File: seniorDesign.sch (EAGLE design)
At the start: 23 parts, among them Q1 mmbt2222, Q2 mmbt2222, Q3 BSS138, U1 TCS34725, X2 ESP-12

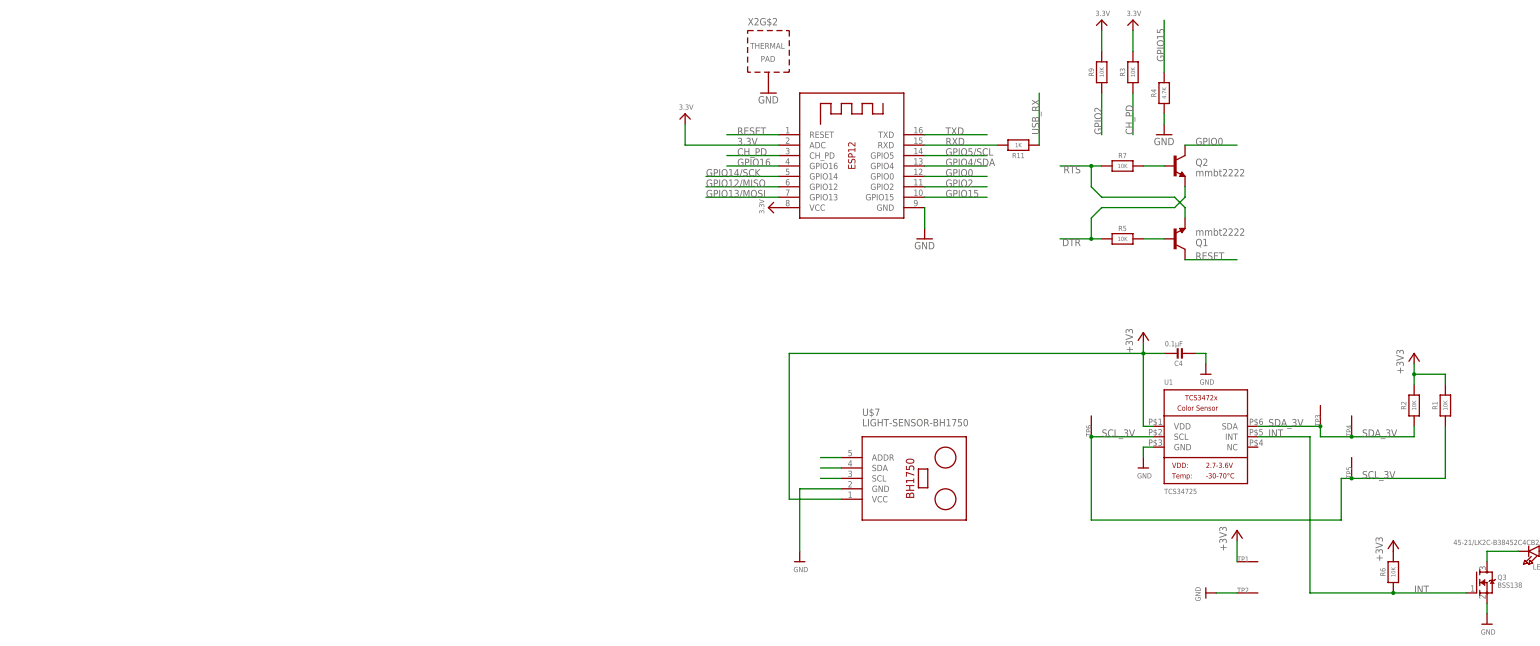
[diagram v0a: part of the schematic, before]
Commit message: Add files via upload
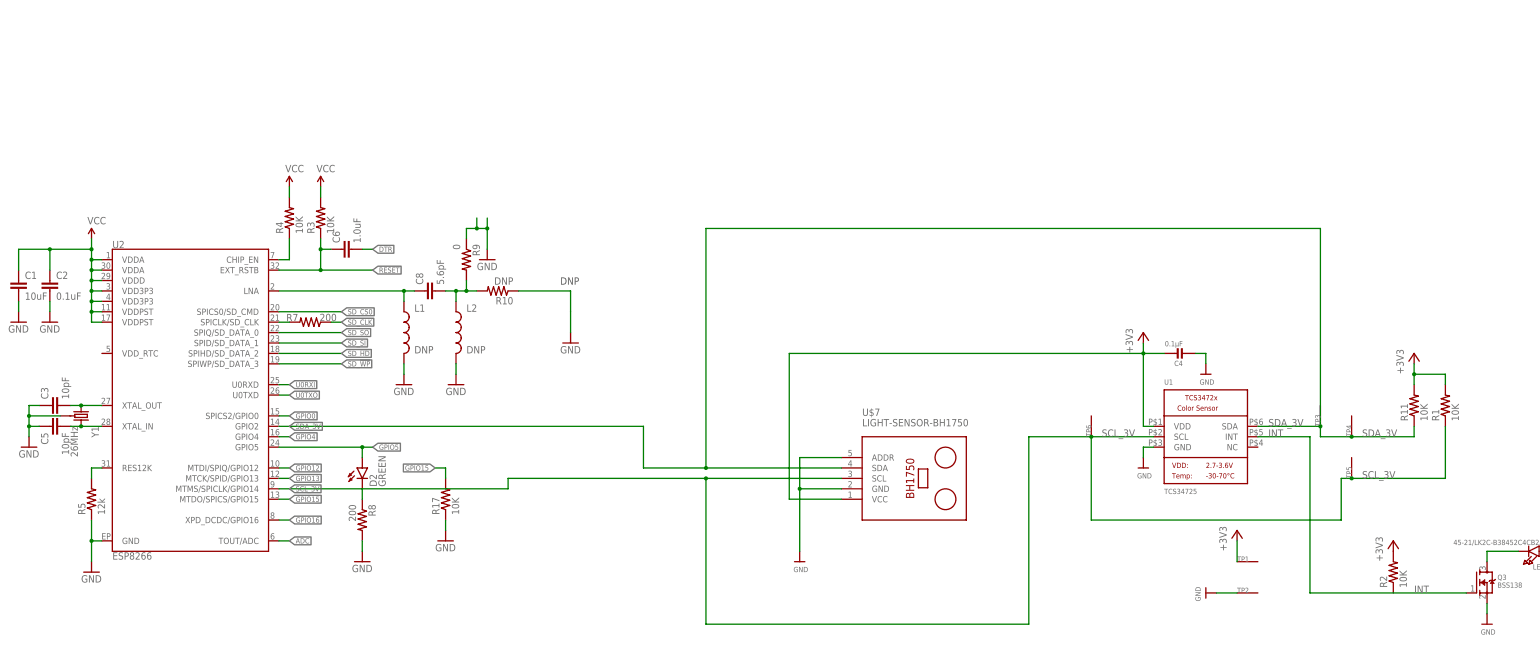
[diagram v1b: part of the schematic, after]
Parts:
- removed Q1, Q2: mmbt2222, SparkFun:TRANSISTOR_NPNSOT23-3
- removed R6: 10K, microbuilder:RESISTOR_0805
- removed X2: ESP-12, microbuilder:ESP-12S
- added C1: 10uF, SparkFun-Capacitors:10UF-6.3V-20%(0603)
- added C2: 0.1uF, SparkFun-Capacitors:0.1UF-25V(+80/-20%)(0603)
- added C3, C5: 10pF, SparkFun-Capacitors:10PF-50V-5%(0603)
- added C6: 1.0uF, SparkFun-Capacitors:1.0UF-16V-10%(0603)
- added C8: 5.6pF, SparkFun-Capacitors:CAP0603-CAP
- added D2: GREEN, SparkFun-LED:LED-GREEN0603
- added L1, L2: DNP, SparkFun-Passives:INDUCTOR0603
- added R10: DNP, SparkFun-Passives:RESISTOR0603-RES
- added R17: 10K, SparkFun-Resistors:10KOHM1/10W1%(0603)0603
- added R8: 200, SparkFun-Resistors:200OHM1/10W1%(0603)
- added U2: ESP8266, SparkFun-RF:ESP8266
- added Y1: 26MHz, things:CRYSTAL-GROUNDED3.2X2.5
- R1, R2: device microbuilder:RESISTOR_0805 -> SparkFun-Resistors:10KOHM1/10W1%(0603)0603
- R11: value 1K -> 10K; device microbuilder:RESISTOR_0603MP -> SparkFun-Resistors:10KOHM1/10W1%(0603)0603
- R3: device microbuilder:RESISTOR_0603_NOOUT -> SparkFun-Resistors:10KOHM1/10W1%(0603)0603
- R4: value 4.7K -> 10K; device microbuilder:RESISTOR_0603_NOOUT -> SparkFun-Resistors:10KOHM1/10W1%(0603)0603
- R5: value 10K -> 12k; device microbuilder:RESISTOR_0603_NOOUT -> SparkFun-Resistors:12KOHM-1/10W-1%(0603)
- R7: value 10K -> 200; device microbuilder:RESISTOR_0603_NOOUT -> SparkFun-Resistors:200OHM1/10W1%(0603)
- R9: value 10K -> 0; device microbuilder:RESISTOR_0603_NOOUT -> SparkFun-Resistors:0OHM1/10W5%(0603)
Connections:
- removed net 3.3V: R3.2, R9.2, X2G$1.ADC, X2G$1.VCC
- removed net CH_PD: R3.1, X2G$1.CH_PD
- removed net GPIO12/MISO: X2G$1.GPIO12
- removed net GPIO13/MOSI: X2G$1.GPIO13
- removed net GPIO14/SCK: X2G$1.GPIO14
- removed net GPIO2: R9.1, X2G$1.GPIO2
- removed net GPIO4/SDA: X2G$1.GPIO4
- removed net GPIO5/SCL: X2G$1.GPIO5
- removed net N$12: Q1.B, R5.2
- removed net N$13: Q2.B, R7.2
- removed net N$2: U$7.SCL
- removed net N$3: U$7.SDA
- removed net N$4: U$7.ADDR
- removed net RTS: Q1.E, R7.1
- removed net RXD: R11.2, X2G$1.RXD
- removed net TXD: X2G$1.TXD
- removed net USB_RX: R11.1
- new net ADC: U2.TOUT/ADC
- new net CHIP_EN: R4.1, U2.CHIP_EN
- new net GPIO12: U2.MTDI/SPIQ/GPIO12
- new net GPIO13: U2.MTCK/SPID/GPIO13
- new net GPIO4: U2.GPIO4
- new net GPIO5: D2.A, U2.GPIO5
- new net LNA: C8.1, L1.1, U2.LNA
- new net N$15: D2.C, R8.1
- new net N$5: R5.2, U2.RES12K
- new net N$6: C5.2, U2.XTAL_IN, Y1.2
- new net N$7: C3.2, U2.XTAL_OUT, Y1.1
- new net N$8: C8.2, L2.1, R10.2, R9.2
- new net N$9: R7.2, U2.SPICLK/SD_CLK
- new net SD_!HD!: U2.SPIHD/SD_DATA_2
- new net SD_!WP!: U2.SPIWP/SD_DATA_3
- new net SD_CLK: R7.1
- new net SD_CS0: U2.SPICS0/SD_CMD
- new net SD_SI: U2.SPID/SD_DATA_1
- new net SD_SO: U2.SPIQ/SD_DATA_0
- new net U0RXI: U2.U0RXD
- new net U0TXO: U2.U0TXD
- new net VCC: C1.1, C2.1, R3.2, R4.2, U2.VDD3P3@3, U2.VDD3P3@4, U2.VDDA@1, U2.VDDA@30, U2.VDDD, U2.VDDPST@11, U2.VDDPST@17
- net +3V3: now also R11.2; no longer R1.2, R6.2
- net DTR: now also C6.2; no longer Q2.E, R5.1
- net GND: now also C1.2, C2.2, C3.1, C5.1, L1.2, L2.2, R10.1, R17.1, R5.1, R8.2, R9.1, U$7.ADDR, U2.GND, Y1.GND; no longer R4.1, X2G$1.GND, X2G$2.TP
- net GPIO0: now also U2.SPICS2/GPIO0; no longer Q2.C, X2G$1.GPIO0
- net GPIO15: now also R17.2, U2.MTDO/SPICS/GPIO15; no longer R4.2, X2G$1.GPIO15
- net GPIO16: now also U2.XPD_DCDC/GPIO16; no longer X2G$1.GPIO16
- net INT: no longer R6.1
- net RESET: now also C6.1, R3.1, U2.EXT_RSTB; no longer Q1.C, X2G$1.RESET
- net SCL_3V: now also U$7.SCL, U2.MTMS/SPICLK/GPIO14; no longer R1.1
- net SDA_3V: now also R11.1, U$7.SDA, U2.GPIO2; no longer R2.1
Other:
- note added: "DNP"
